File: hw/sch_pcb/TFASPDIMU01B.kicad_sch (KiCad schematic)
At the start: 26 parts, among them J1 SM07B-GHS-TB, U1 SDP3x, U2 ICM-20948, U4 MIC5504-3.3YM5-TR, U5 MIC5504-1.8YM5-TR, U6 TXS0108EPW

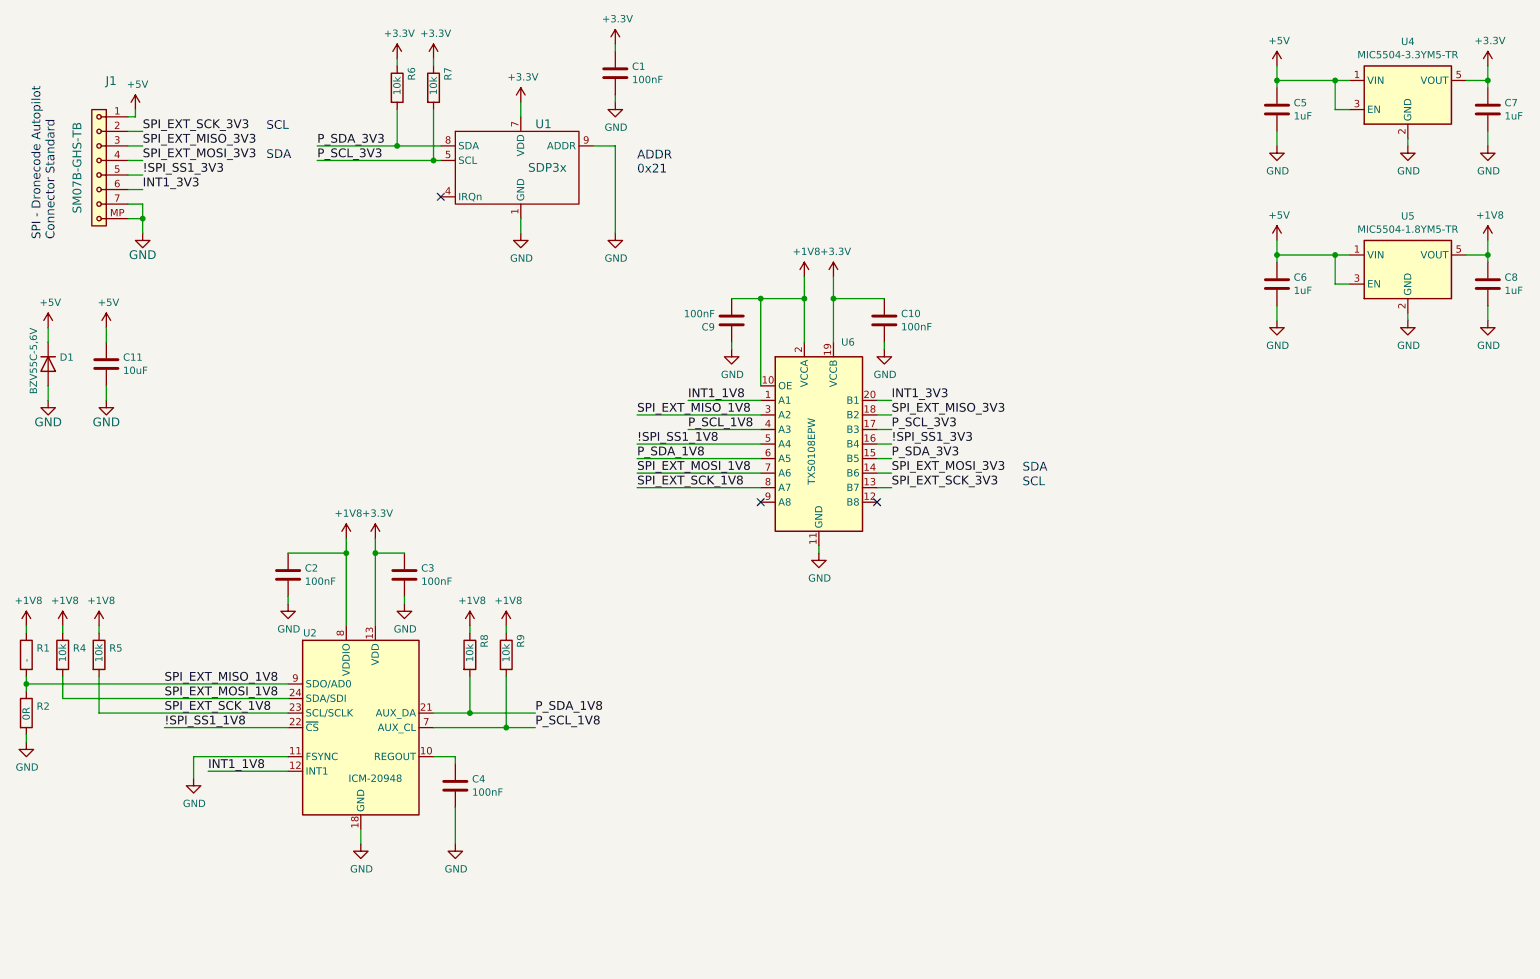
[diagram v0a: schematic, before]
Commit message: Edit schema
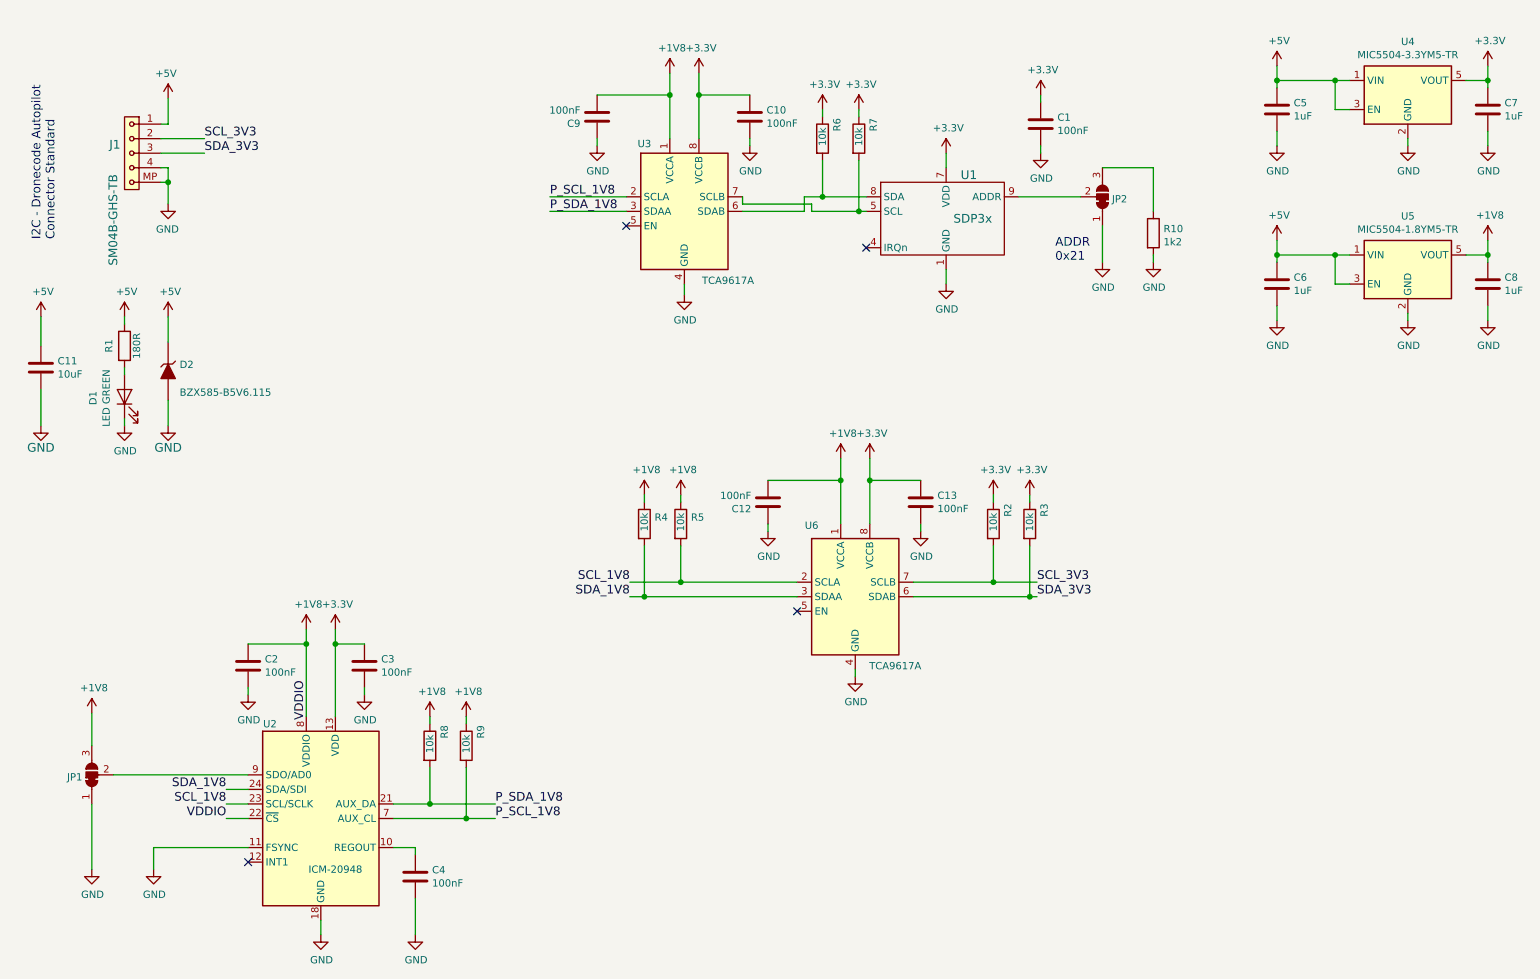
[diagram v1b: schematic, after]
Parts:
- removed D1: BZV55C-5,6V, Diode_SMD:D_MiniMELF, symbol Device:D
- removed J1: SM07B-GHS-TB, Connector_JST:JST_GH_SM07B-GHS-TB_1x07-1MP_P1.25mm_Horizontal, symbol MLAB_CONNECTORS_JST:SM07B-GHS-TB
- removed U6: TXS0108EPW, Package_SO:TSSOP-20_4.4x6.5mm_P0.65mm, symbol Logic_LevelTranslator:TXS0108EPW
- added C12, C13: 100nF, Mlab_R:SMD-0603, symbol Device:C
- added D1: LED GREEN, Mlab_D:LED_1206, symbol Device:LED
- added D2: BZX585-B5V6.115, Diode_SMD:D_SOD-523, symbol MLAB_D:D_ZENER
- added J1: SM04B-GHS-TB, Connector_JST:JST_GH_SM04B-GHS-TB_1x04-1MP_P1.25mm_Horizontal, symbol MLAB_CONNECTORS_JST:SM04B-GHS-TB
- added JP1, JP2: SolderJumper_3_Bridged12, symbol Jumper:SolderJumper_3_Bridged12
- added R10: 1k2, symbol Device:R
- added R3: 10k, Mlab_R:SMD-0603, symbol Device:R
- added U3, U6: TCA9617A, Package_SO:TSSOP-8_3x3mm_P0.65mm, symbol Interface:TCA9800
- R1: value - -> 180R; UST_ID (none) -> 5c70984512875079b91f8957
- R2: value 0R -> 10k; UST_ID 5c70984512875079b91f896b -> 5c70984612875079b91f899f
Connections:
- net !SPI_SS1_1V8 is gone; now on net +1V8: U2.22 (~CS)
- net +1V8: now also C12.2, JP1.3 (B), U3.1 (VCCA), U6.1 (VCCA); no longer R1.1
- net +3V3: now also R2.1, C13.1, R3.1, U3.8 (VCCB), U6.8 (VCCB)
- net +5V: now also R1.1, D2.1 (K), J1.1
- net GND: now also C12.1, C13.2, D1.1 (K), D2.2 (A), J1.4, J1.MP, JP1.1 (A), JP2.1 (A), R10.2, U3.4 (GND), U6.4 (GND); no longer R2.2, U1.9 (ADDR)
- net P_SCL_1V8: now also U3.2 (SCLA)
- net P_SDA_1V8: now also U3.3 (SDAA)
- net INT1_1V8: no longer names the net of U2.12 (INT1)
- net P_SCL_3V3: no longer names the net of R7.2, U1.5 (SCL)
- net P_SCL_3V3: now also U3.7 (SCLB)
- net P_SDA_3V3: no longer names the net of R6.2, U1.8 (SDA)
- net P_SDA_3V3: now also U3.6 (SDAB)
- removed net SPI_EXT_MISO_1V8: R1.2, R2.1, U2.9 (SDO/AD0)
- net SPI_EXT_MOSI_1V8 renamed SDA_1V8
- net SDA_1V8: now also U6.3 (SDAA)
- net SPI_EXT_SCK_1V8 renamed SCL_1V8
- net SCL_1V8: now also U6.2 (SCLA)
- new net: JP1.2 (C), U2.9 (SDO/AD0)
- new net: JP2.2 (C), U1.9 (ADDR)
- new net: JP2.3 (B), R10.1
- new net: D1.2 (A), R1.2
- new net SCL_3V3: J1.2, R2.2, U6.7 (SCLB)
- new net SDA_3V3: J1.3, R3.2, U6.6 (SDAB)
- no-connect marks 3 -> 4
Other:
- note added: "I2C - Dronecode Autopilot Connector Standard"
- note removed: "SCL"
- note removed: "SDA"
- note removed: "SPI - Dronecode Autopilot Connector Standard"
- moved on the sheet: C1, C10, C11, C2, C3, C4, C9, R4, R5, R6, R7, R8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
